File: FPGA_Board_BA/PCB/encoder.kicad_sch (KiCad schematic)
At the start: 1 part, among them J1101 Molex_Mini_Fit_Jr_2x08pin

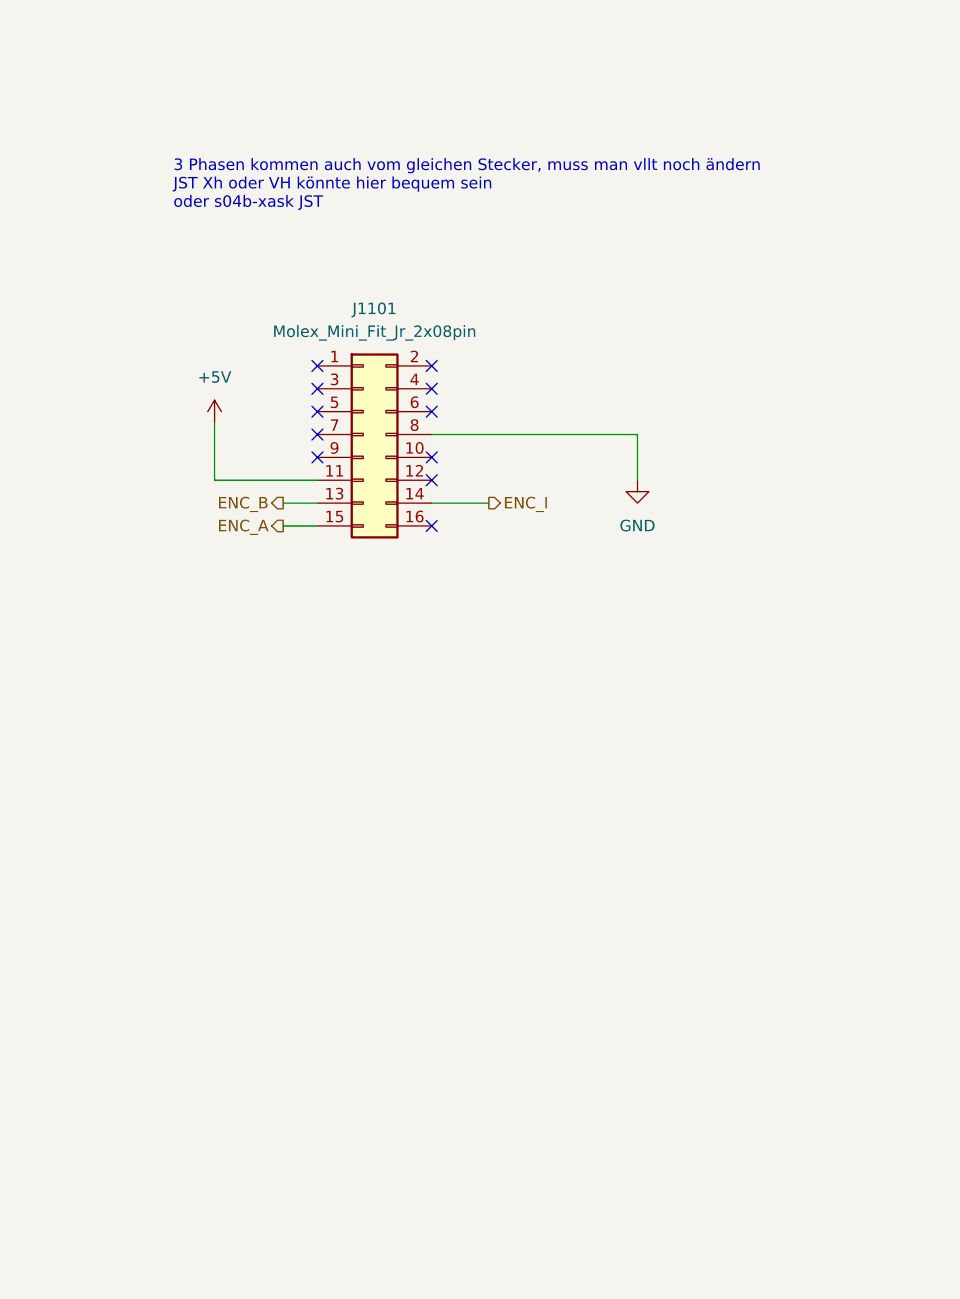
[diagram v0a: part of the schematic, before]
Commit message: lots of work
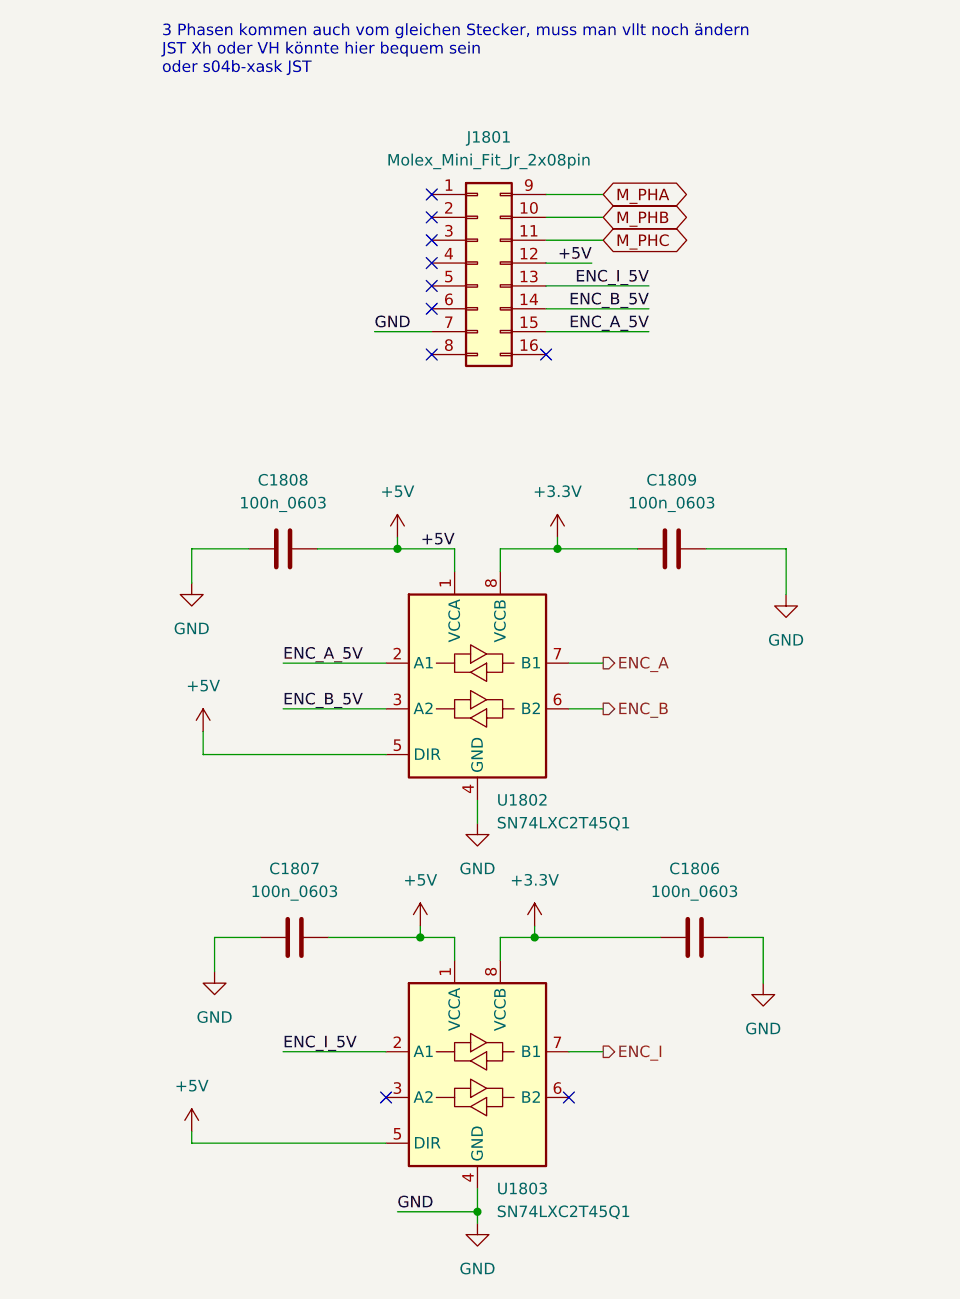
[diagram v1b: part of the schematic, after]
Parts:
- removed J1101: Molex_Mini_Fit_Jr_2x08pin, MYLIB_Misc:Molex_2x8pin_vertical_tht, symbol MYLIB_Misc:Molex_Mini_Fit_Jr_2x08
- added C1806, C1807, C1808, C1809: 100n_0603, WLIB_Capacitor:C_0603, symbol WLIB_C:100n_0603
- added J1801: Molex_Mini_Fit_Jr_2x08pin, MYLIB_Misc:Molex_2x8pin_vertical_tht, symbol MYLIB_Misc:Molex_Mini_Fit_Jr_2x08
- added U1802, U1803: SN74LXC2T45Q1, MYLIB_Misc:SN74LXC2T45QDCURQ1, symbol MYLIB_Misc:SN74LXC2T45Q1
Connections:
- net +5V: now also C1807.2, C1808.2, J1801.12 (Pin_12), U1802.1 (VCCA), U1802.5 (DIR), U1803.1 (VCCA), U1803.5 (DIR)
- net ENC_A: now also U1802.7 (B1)
- net ENC_B: now also U1802.6 (B2)
- net ENC_I: now also U1803.7 (B1)
- net GND: now also C1806.2, C1807.1, C1808.1, C1809.2, J1801.7 (Pin_7), U1802.4 (GND), U1803.4 (GND)
- new net +3.3V: C1806.1, C1809.1, U1802.8 (VCCB), U1803.8 (VCCB)
- new net ENC_A_5V: J1801.15 (Pin_15), U1802.2 (A1)
- new net ENC_B_5V: J1801.14 (Pin_14), U1802.3 (A2)
- new net ENC_I_5V: J1801.13 (Pin_13), U1803.2 (A1)
- new net M_PHA: J1801.9 (Pin_9)
- new net M_PHB: J1801.10 (Pin_10)
- new net M_PHC: J1801.11 (Pin_11)
- no-connect marks 11 -> 10
